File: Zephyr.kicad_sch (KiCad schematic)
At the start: 44 parts, among them J1 Conn_02x03_Counter_Clockwise, J11 Conn_01x03, J13 Conn_01x03, J14 Conn_01x06, J15 Micro_SD_Card, Q1 MMBT3904, Q2 MMBT3904, SW4 SW_Push, U1 STM32F405RGT6, U9 W25Q128JVS, Y1 32.768KHz 12.5pF, Y2 8MHz 12pF

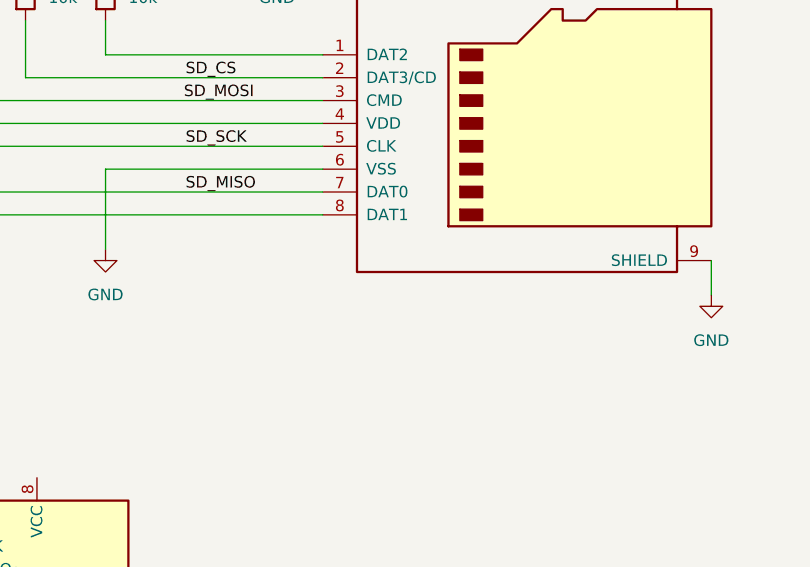
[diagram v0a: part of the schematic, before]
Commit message: SD card
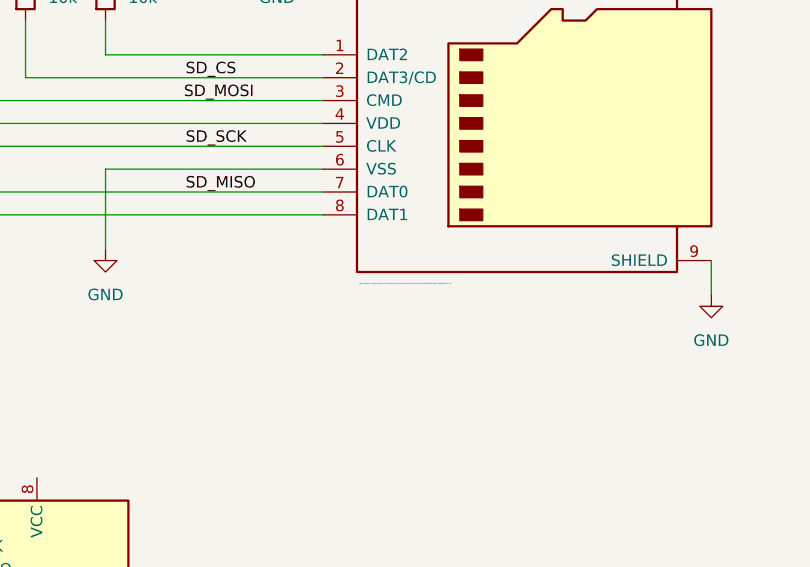
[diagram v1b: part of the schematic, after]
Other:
- note added: "https://github.com/sbcshop/MicroSD-Breakout/blob/main/Hardware%20Files/SCH%20SD%20CARD%20BREAKOUT.pdf"
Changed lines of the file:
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@@
 	(generator_version "9.0")
 	(paper "A3")
+	(text "https://github.com/sbcshop/MicroSD-Breakout/blob/main/Hardware%20Files/SCH%20SD%20CARD%20BREAKOUT.pdf"
+		(exclude_from_sim no)
+		(at 346.964 171.704 0)
+		(effects
+			(font
+				(size 0.127 0.127)
+			)
+		)
+	)
 	(text "C51927445"
 		(exclude_from_sim no)
